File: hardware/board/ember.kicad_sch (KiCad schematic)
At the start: 133 parts, among them Q2 2SC1815_C727146, Q3 IRF1018ESTRLPBF, SW1 EC11E18244A5, SW2 SW_Push, SW3 SW_Push, U1 TPS25730D, U10 NT3H2111W0FHKH, U11 DB128L-5.08-2P-BK-S, U12 MAX31865xTP, U13 MAX6675ISA+T, U14 DB128L-5.08-3P-BK-S, U2 LM22676MR-ADJ, U3 TPD6S300A, U4 DB128L-5.08-2P-BK-S, U5 INA226, U6 TMP119AIYBGR, U7 TLP183(GRH-TPL,E(T, U8 W25Q256JVEIQTR, U9 STM32WB55REVx, X1 XL7EL89CKI-111YLC-32M, X2 X201232768KJD2SI

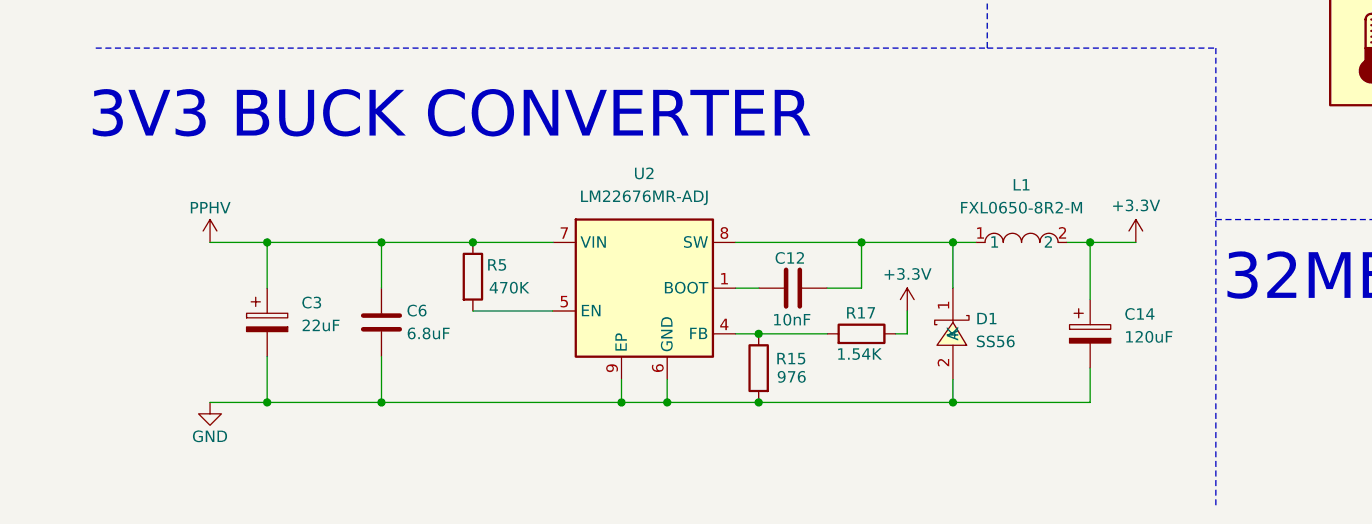
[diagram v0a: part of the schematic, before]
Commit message: changed buck
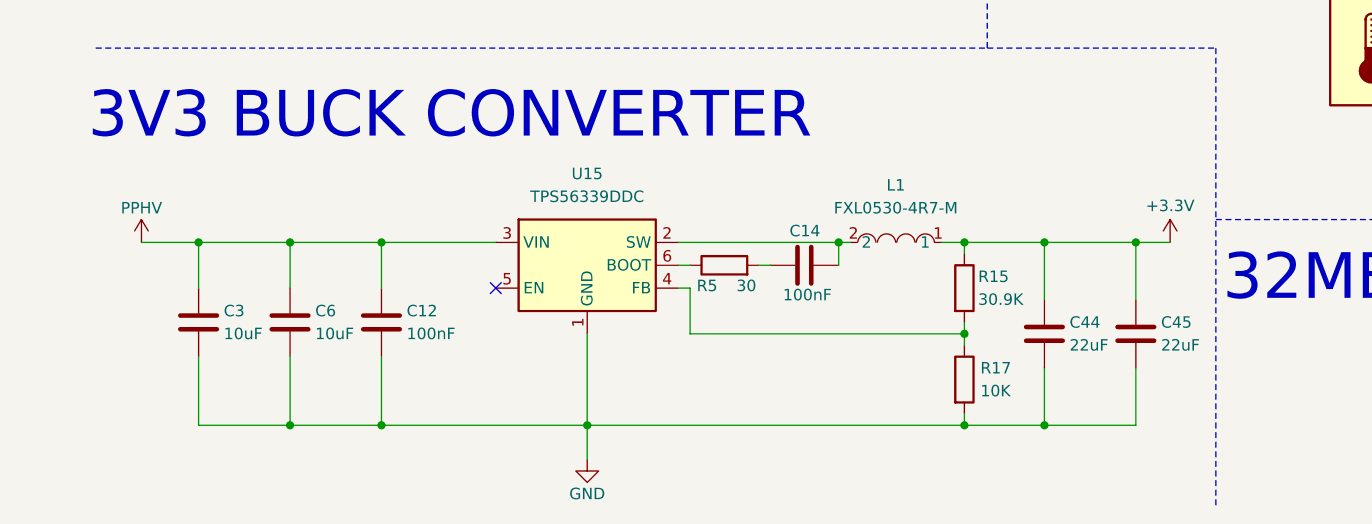
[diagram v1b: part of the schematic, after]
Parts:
- removed C14: 120uF, Capacitor_SMD:CP_Elec_6.3x7.7, symbol Device:C_Polarized
- removed C3: 22uF, Capacitor_SMD:CP_Elec_6.3x5.4, symbol Device:C_Polarized
- removed D1: SS56, lcsc:SMA_L4.3-W2.6-LS5.2-RD, symbol lcsc:SS56
- removed L1: FXL0650-8R2-M, lcsc:IND-SMD_L7.0-W6.6_FXL0650, symbol lcsc:FXL0650-8R2-M
- removed U2: LM22676MR-ADJ, Package_SO:TI_SO-PowerPAD-8, symbol Regulator_Switching:LM22676MR-ADJ
- added C14: 100nF, Capacitor_SMD:C_0402_1005Metric, symbol Device:C
- added C3: 10uF, Capacitor_SMD:C_0805_2012Metric, symbol Device:C
- added C44, C45: 22uF, Capacitor_SMD:C_0805_2012Metric, symbol Device:C
- added L1: FXL0530-4R7-M, lcsc:IND-SMD_L5.4-W5.2_FXL0530, symbol lcsc:FXL0530-4R7-M
- added U15: TPS56339DDC, Package_TO_SOT_SMD:SOT-23-6, symbol Regulator_Switching:TPS56339DDC
- C12: value 10nF -> 100nF; footprint Capacitor_SMD:C_0402_1005Metric -> Capacitor_SMD:C_0603_1608Metric
- C6: value 6.8uF -> 10uF; footprint Capacitor_SMD:C_0603_1608Metric -> Capacitor_SMD:C_0805_2012Metric
- R15: value 976 -> 30.9K
- R17: value 1.54K -> 10K
- R5: value 470K -> 30; footprint Resistor_SMD:R_0603_1608Metric -> Resistor_SMD:R_0402_1005Metric
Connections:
- net +3.3V: now also R15.1, C44.1, C45.1, L1.1; no longer R17.1
- net GND: now also C12.2, R17.2, C3.2, C44.2, C45.2, U15.1 (GND); no longer R15.2
- net PPHV: now also C12.1, C3.1, U15.3 (VIN); no longer R5.1
- net at R5.2: now also C14.1
- new net: R5.1, U15.6 (BOOT)
- new net: C14.2, L1.2, U15.2 (SW)
- new net: R15.2, R17.1, U15.4 (FB)
- no-connect marks 16 -> 17
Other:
- moved on the sheet: C6
